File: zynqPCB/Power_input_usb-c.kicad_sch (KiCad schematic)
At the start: 6 parts, among them J1 USB4105-GF-A-120

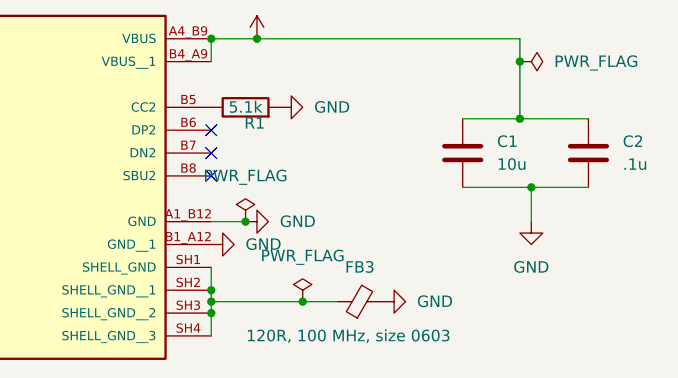
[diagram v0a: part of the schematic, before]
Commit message: Ferrite Bead
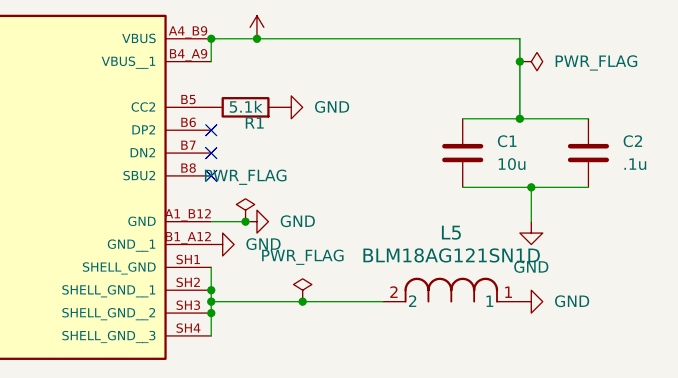
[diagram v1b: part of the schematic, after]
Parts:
- removed FB3: 120R, 100 MHz, size 0603, Inductor_SMD:L_0603_1608Metric, symbol Device:Ferrite_Bead_Small
- added L5: BLM18AG121SN1D, DFTcustom:IND_BLM18_0603_MUR-L, symbol Ferrite_Bead:BLM18AG121SN1D
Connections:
- net GND: now also L5.1
- net at J1.SH1 (SHELL_GND), J1.SH2 (SHELL_GND__1), J1.SH3 (SHELL_GND__2)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: now also L5.2
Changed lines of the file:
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@@
+	(wire
+		(pts
+			(xy 138.43 116.84) (xy 129.54 116.84)
+		)
+		(stroke
+			(width 0)
+			(type default)
+		)
+	)
 	(wire
 		(pts
@@
 		)
 	)
-	(wire
-		(pts
-			(xy 129.54 116.84) (xy 133.35 116.84)
-		)
-		(stroke
-			(width 0)
-			(type default)
-		)
-	)
 	(symbol
 		(lib_id "Device:C")
@@
 	)
 	(symbol
-		(lib_id "Device:Ferrite_Bead_Small")
-		(at 135.89 116.84 90)
-		(unit 1)
-		(body_style 1)
-		(exclude_from_sim no)
-		(in_bom yes)
-		(on_board yes)
-		(in_pos_files yes)
-		(dnp no)
-		(property "Reference" "FB3"
-			(at 135.89 113.03 90)
-			(show_name no)
-			(do_not_autoplace no)
-			(effects
-				(font
-					(size 1.27 1.27)
-				)
-			)
-		)
-		(property "Value" "120R, 100 MHz, size 0603"
-			(at 134.62 120.65 90)
-			(show_name no)
-			(do_not_autoplace no)
-			(effects
-				(font
-					(size 1.27 1.27)
-				)
-			)
-		)
-		(property "Footprint" "Inductor_SMD:L_0603_1608Metric"
-			(at 135.89 118.618 90)
-			(hide yes)
-			(show_name no)
-			(do_not_autoplace no)
-			(effects
-				(font
-					(size 1.27 1.27)
-				)
-			)
-		)
-		(property "Datasheet" ""
-			(at 135.89 116.84 0)
-			(hide yes)
-			(show_name no)
-			(do_not_autoplace no)
-			(effects
-				(font
-					(size 1.27 1.27)
+		(lib_id "Ferrite_Bead:BLM18AG121SN1D")
+		(at 138.43 116.84 0)
+		(unit 1)
+		(body_style 1)
+		(exclude_from_sim no)
+		(in_bom yes)
+		(on_board yes)
+		(in_pos_files yes)
+		(dnp no)
+		(fields_autoplaced yes)
+		(property "Reference" "L5"
+			(at 146.05 109.22 0)
+			(show_name no)
+			(do_not_autoplace no)
+			(effects
+				(font
+					(size 1.524 1.524)
+				)
+			)
+		)
+		(property "Value" "BLM18AG121SN1D"
+			(at 146.05 111.76 0)
+			(show_name no)
+			(do_not_autoplace no)
+			(effects
+				(font
+					(size 1.524 1.524)
+				)
+			)
+		)
+		(property "Footprint" "DFTcustom:IND_BLM18_0603_MUR-L"
+			(at 138.43 116.84 0)
+			(hide yes)
+			(show_name no)
+			(do_not_autoplace no)
+			(effects
+				(font
+					(size 1.27 1.27)
+					(italic yes)
+				)
+			)
+		)
+		(property "Datasheet" "BLM18AG121SN1D"
+			(at 138.43 116.84 0)
+			(hide yes)
+			(show_name no)
+			(do_not_autoplace no)
+			(effects
+				(font
+					(size 1.27 1.27)
+					(italic yes)
 				)
 			)
 		)
 		(property "Description" ""
-			(at 135.89 116.84 0)
-			(show_name no)
-			(do_not_autoplace no)
-			(effects
-				(font
-					(size 1.27 1.27)
-				)
-			)
-		)
-		(property "MFR" "Murata Electronics"
-			(at 295.91 355.6 0)
-			(hide yes)
-			(show_name no)
-			(do_not_autoplace no)
-			(effects
-				(font
-					(size 1.27 1.27)
-				)
-			)
-		)
-		(property "MPN" "BLM18AG121SN1D"
-			(at 295.91 355.6 0)
-			(hide yes)
-			(show_name no)
-			(do_not_autoplace no)
-			(effects
-				(font
-					(size 1.27 1.27)
-				)
-			)
-		)
-		(property "SPR" "Digikey"
-			(at 295.91 355.6 0)
-			(hide yes)
-			(show_name no)
-			(do_not_autoplace no)
-			(effects
-				(font
-					(size 1.27 1.27)
-				)
-			)
-		)
-		(property "SPN" "490-1011-1-ND"
-			(at 295.91 355.6 0)
-			(hide yes)
-			(show_name no)
-			(do_not_autoplace no)
-			(effects
-				(font
-					(size 1.27 1.27)
-				)
-			)
-		)
-		(property "SPURL" "-"
-			(at 295.91 355.6 0)
+			(at 138.43 116.84 0)
 			(hide yes)
 			(show_name no)
@@
 			(project "DFTBoard"
 				(path "/49eba173-d38c-4d05-b21c-b4a14c4948c2/f959ad9d-3c11-4f00-a0f3-569c86969599"
-					(reference "FB3")
+					(reference "L5")
 					(unit 1)
 				)
@@
 	(symbol
 		(lib_id "power:GND")
-		(at 138.43 116.84 90)
+		(at 153.67 116.84 90)
 		(unit 1)
 		(body_style 1)
@@
 		(fields_autoplaced yes)
 		(property "Reference" "#PWR024"
-			(at 144.78 116.84 0)
+			(at 160.02 116.84 0)
 			(hide yes)
 			(show_name no)
@@
 		)
 		(property "Value" "GND"
-			(at 142.24 116.8399 90)
+			(at 157.48 116.8399 90)
 			(show_name no)
 			(do_not_autoplace no)
@@
 		)
 		(property "Footprint" ""
-			(at 138.43 116.84 0)
-			(hide yes)
-			(show_name no)
-			(do_not_autoplace no)
-			(effects
-				(font
-					(size 1.27 1.27)
-				)
-			)
-		)
-		(property "Datasheet" ""
-			(at 138.43 116.84 0)
+			(at 153.67 116.84 0)
+			(hide yes)
+			(show_name no)
+			(do_not_autoplace no)
+			(effects
+				(font
+					(size 1.27 1.27)
+				)
+			)
+		)
+		(property "Datasheet" ""
+			(at 153.67 116.84 0)
 			(hide yes)
 			(show_name no)
@@
 		)
 		(property "Description" "Power symbol creates a global label with name \"GND\" , ground"
-			(at 138.43 116.84 0)
-			(hide yes)
-			(show_name no)
+			(at 153.67 116.84 0)
+			(hide yes)
+			(show_name no)
